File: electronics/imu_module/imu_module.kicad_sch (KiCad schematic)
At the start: 32 parts, among them J1 Conn_01x06_Male, J2 Conn_01x03_Male, J3 Conn_01x04, J4 Conn_01x04, U1 ESP32-WROOM-32U, U2 BMI088, U3 SN74LV1T34DBVR, U4 SP485, U5 AP2114HA-3.3TRG1

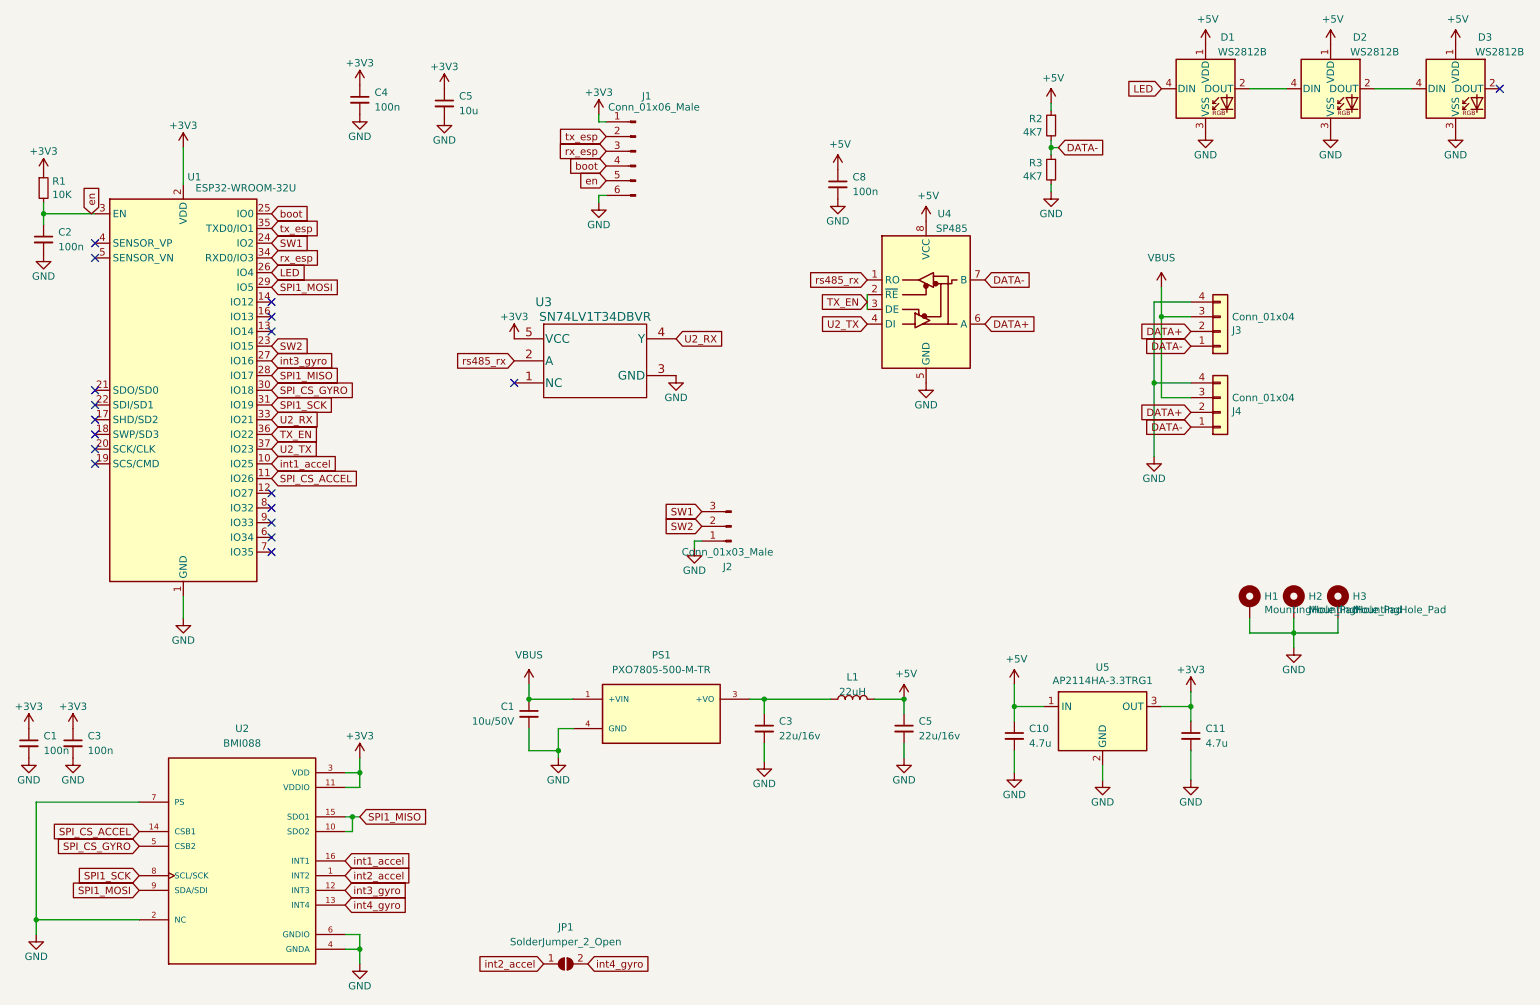
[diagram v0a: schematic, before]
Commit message: library updates
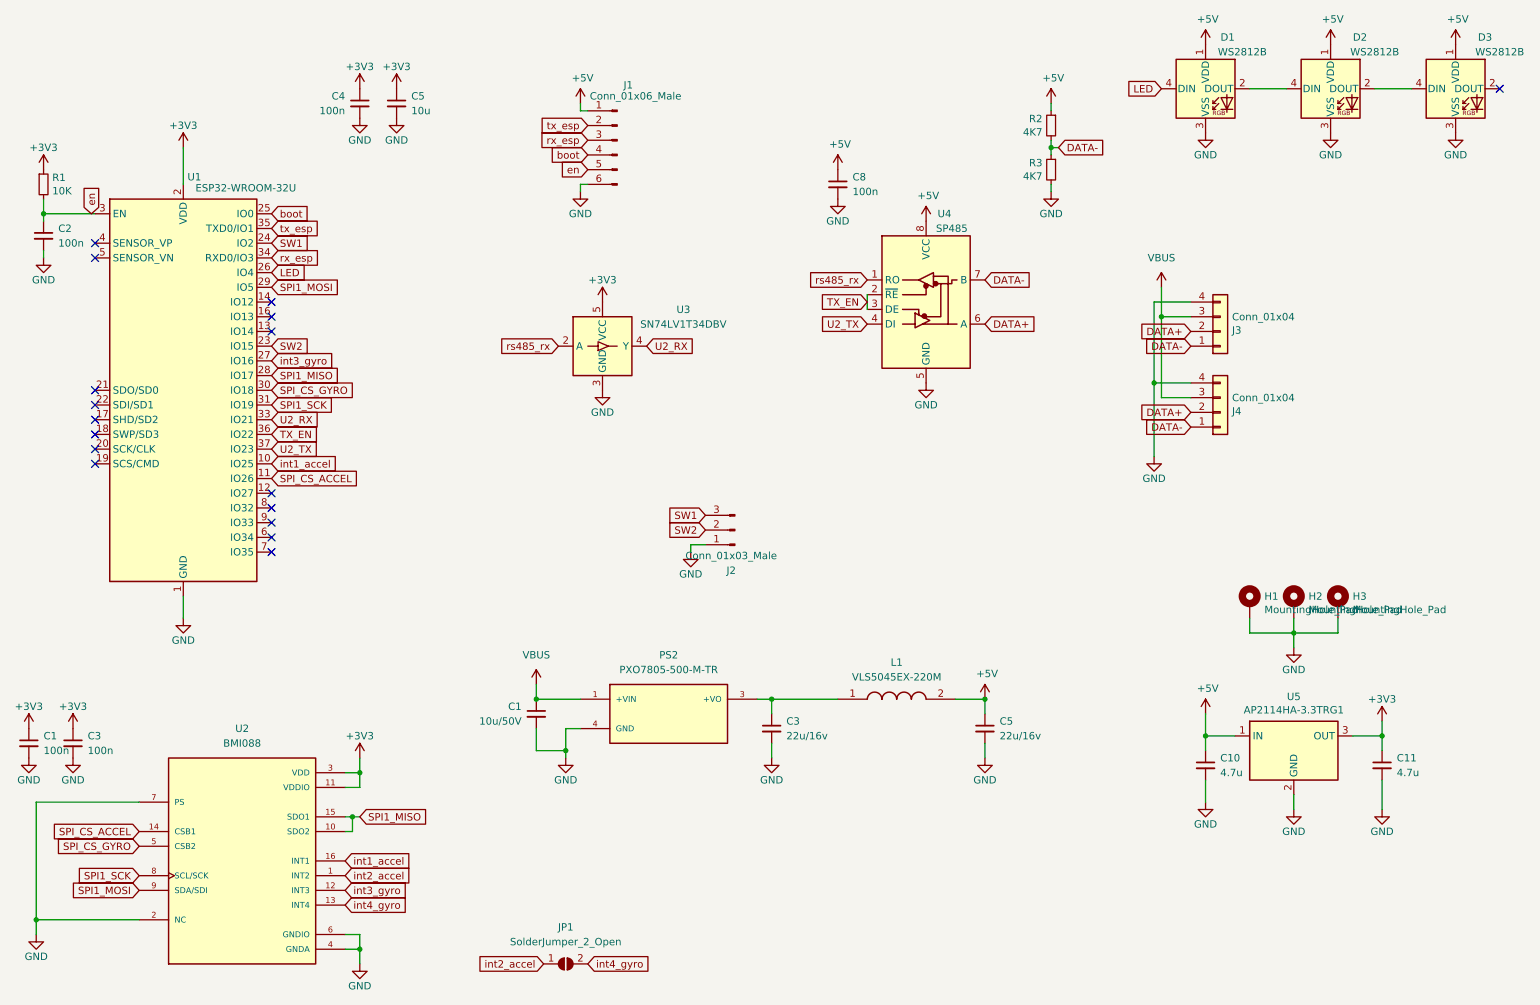
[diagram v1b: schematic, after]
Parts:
- removed L1: 22uH, lib:VLS5045EX330M, symbol Device:L
- removed PS1: PXO7805-500-M-TR, lib:CONV_PXO7805-500-M-TR, symbol PXO7805-500-M-TR:PXO7805-500-M-TR
- removed U3: SN74LV1T34DBVR, bitbots:SN74LV1T34DBVR, symbol SN74LV1T34DBVR:SN74LV1T34DBVR
- added L1: VLS5045EX-220M, lib:VLS5045EX330M, symbol VLS5045EX-220M:VLS5045EX-220M
- added PS2: PXO7805-500-M-TR, lib:PXO7805-500-M-TR, symbol PXO7805-500-M-TR:PXO7805-500-M-TR
- added U3: SN74LV1T34DBV, Package_TO_SOT_SMD:SOT-23-5, symbol Logic_LevelTranslator:SN74LV1T34DBV
- J1: footprint bitbots:testpoint_01x06 -> bitbots:esp32_pogo_programmer
- U2: footprint lib:PQFN50P450X300X100-16N -> lib:BMI088; DESCRIPTION Accelerometer, Gyroscope, 6 Axis Sensor I²C, SPI Output -> (none)
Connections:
- net +3V3: now also U3.5 (VCC); no longer J1.1 (Pin_1)
- net +5V: now also J1.1 (Pin_1), L1.2
- net GND: now also PS2.4 (GND), U3.3 (GND)
- net U2_RX: now also U3.4 (Y)
- net VBUS: now also PS2.1 (+VIN)
- net rs485_rx: now also U3.2 (A)
- net at C3.1: now also L1.1, PS2.3 (+VO)
- no-connect marks 18 -> 17
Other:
- moved on the sheet: C1, C10, C11, C2, C3, C4, C5, J1, J2, R1, U5

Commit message: prep for production
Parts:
- C1: LCSC Part # C1525 -> C13585
- C1, C2, C3, C4, C8: LCSC Part # C1525 -> C49678
- C10, C11: LCSC Part # C1525 -> C29823
- C3, C5: LCSC Part # C1525 -> C12891
- C5: LCSC Part # C1525 -> C15850
- H1, H2, H3, J2, JP1: now left out of the parts list
- J1: footprint bitbots:esp32_pogo_programmer -> lib:esp32_pogo_programmer; now left out of the parts list
- R1: LCSC Part # (none) -> C17414
- R2, R3: LCSC Part # (none) -> C17673
- U1: LCSC Part # (none) -> C3013937
- U2: LCSC Part # (none) -> C194919
- U3: LCSC Part # (none) -> C100024
- U4: LCSC Part # (none) -> C6855
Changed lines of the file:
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@@
 			)
 		)
-		(property "LCSC Part #" "C1525"
+		(property "LCSC Part #" "C49678"
 			(at 27.94 55.88 0)
 			(effects
@@
 			)
 		)
-		(property "LCSC Part #" "C1525"
+		(property "LCSC Part #" "C49678"
 			(at 165.1 46.99 0)
 			(effects
@@
 			)
 		)
-		(property "LCSC Part #" "C1525"
+		(property "LCSC Part #" "C15850"
 			(at 88.9 33.02 0)
 			(effects
@@
 			)
 		)
+		(property "LCSC Part #" "C17414"
+			(at 27.94 46.99 0)
+			(effects
+				(font
+					(size 1.27 1.27)
+				)
+				(hide yes)
+			)
+		)
 		(pin "1"
 		)
@@
 		(unit 1)
 		(exclude_from_sim no)
-		(in_bom yes)
+		(in_bom no)
 		(on_board yes)
 		(dnp no)
@@
 			)
 		)
-		(property "Footprint" "bitbots:esp32_pogo_programmer"
+		(property "Footprint" "lib:esp32_pogo_programmer"
 			(at 127 39.37 0)
 			(effects
@@
 			)
 		)
+		(property "LCSC Part #" "C3013937"
+			(at 52.07 82.55 0)
+			(effects
+				(font
+					(size 1.27 1.27)
+				)
+				(hide yes)
+			)
+		)
 		(pin "1"
 		)
@@
 			)
 		)
+		(property "LCSC Part #" "C6855"
+			(at 180.34 66.04 0)
+			(effects
+				(font
+					(size 1.27 1.27)
+				)
+				(hide yes)
+			)
+		)
 		(pin "1"
 		)
@@
 			)
 		)
-		(property "LCSC Part #" "C1525"
+		(property "LCSC Part #" "C49678"
 			(at 82.55 33.02 0)
 			(effects
@@
 		(unit 1)
 		(exclude_from_sim no)
-		(in_bom yes)
+		(in_bom no)
 		(on_board yes)
 		(dnp no)
@@
 		(unit 1)
 		(exclude_from_sim no)
-		(in_bom yes)
+		(in_bom no)
 		(on_board yes)
 		(dnp no)
@@
 		(unit 1)
 		(exclude_from_sim no)
-		(in_bom yes)
+		(in_bom no)
 		(on_board yes)
 		(dnp no)
@@
 			)
 		)
-		(property "LCSC Part #" "C1525"
+		(property "LCSC Part #" "C29823"
 			(at 259.08 147.32 0)
 			(effects
@@
 			)
 		)
-		(property "LCSC Part #" "C1525"
+		(property "LCSC Part #" "C29823"
 			(at 228.6 147.32 0)
 			(effects
@@
 			)
 		)
+		(property "LCSC Part #" "C17673"
+			(at 201.93 36.83 0)
+			(effects
+				(font
+					(size 1.27 1.27)
+				)
+				(hide yes)
+			)
+		)
 		(pin "1"
 		)
@@
 			)
 		)
-		(property "LCSC Part #" "C1525"
+		(property "LCSC Part #" "C13585"
 			(at 113.03 138.43 0)
 			(effects
@@
 			)
 		)
+		(property "LCSC Part #" "C194919"
+			(at 62.23 163.83 0)
+			(effects
+				(font
+					(size 1.27 1.27)
+				)
+				(hide yes)
+			)
+		)
 		(pin "2"
 		)
@@
 			)
 		)
-		(property "LCSC Part #" "C1525"
+		(property "LCSC Part #" "C12891"
 			(at 190.5 140.97 0)
 			(effects
@@
 		(unit 1)
 		(exclude_from_sim no)
-		(in_bom yes)
+		(in_bom no)
 		(on_board yes)
 		(dnp no)
@@
 		(unit 1)
 		(exclude_from_sim no)
-		(in_bom yes)
+		(in_bom no)
 		(on_board yes)
 		(dnp no)
@@
 			)
 		)
+		(property "LCSC Part #" "C100024"
+			(at 124.46 74.93 0)
+			(effects
+				(font
+					(size 1.27 1.27)
+				)
+				(hide yes)
+			)
+		)
 		(pin "4"
 		)
@@
 			)
 		)
-		(property "LCSC Part #" "C1525"
+		(property "LCSC Part #" "C49678"
 			(at 33.02 143.51 0)
 			(effects
@@
 			)
 		)
-		(property "LCSC Part #" "C1525"
+		(property "LCSC Part #" "C12891"
 			(at 153.67 140.97 0)
 			(effects
@@
 			)
 		)
+		(property "LCSC Part #" "C17673"
+			(at 201.93 44.45 0)
+			(effects
+				(font
+					(size 1.27 1.27)
+				)
+				(hide yes)
+			)
+		)
 		(pin "1"
 		)
@@
 			)
 		)
-		(property "LCSC Part #" "C1525"
+		(property "LCSC Part #" "C49678"
 			(at 25.4 143.51 0)
 			(effects
